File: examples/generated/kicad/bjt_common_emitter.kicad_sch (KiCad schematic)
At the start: 6 parts, among them Q1 2N3904

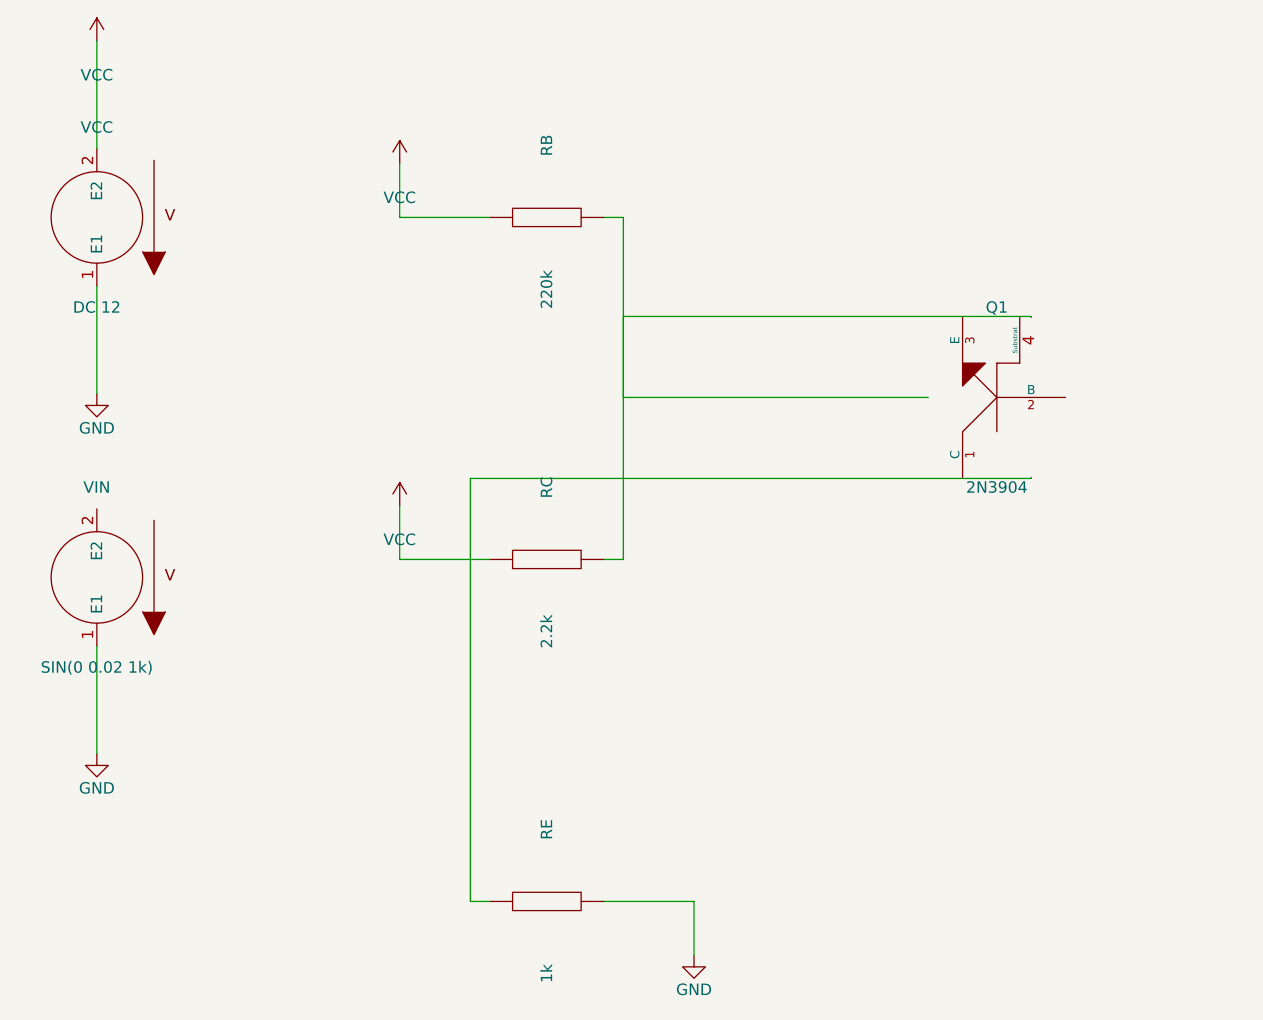
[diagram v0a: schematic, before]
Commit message: Attempt to fix more terminal issues.
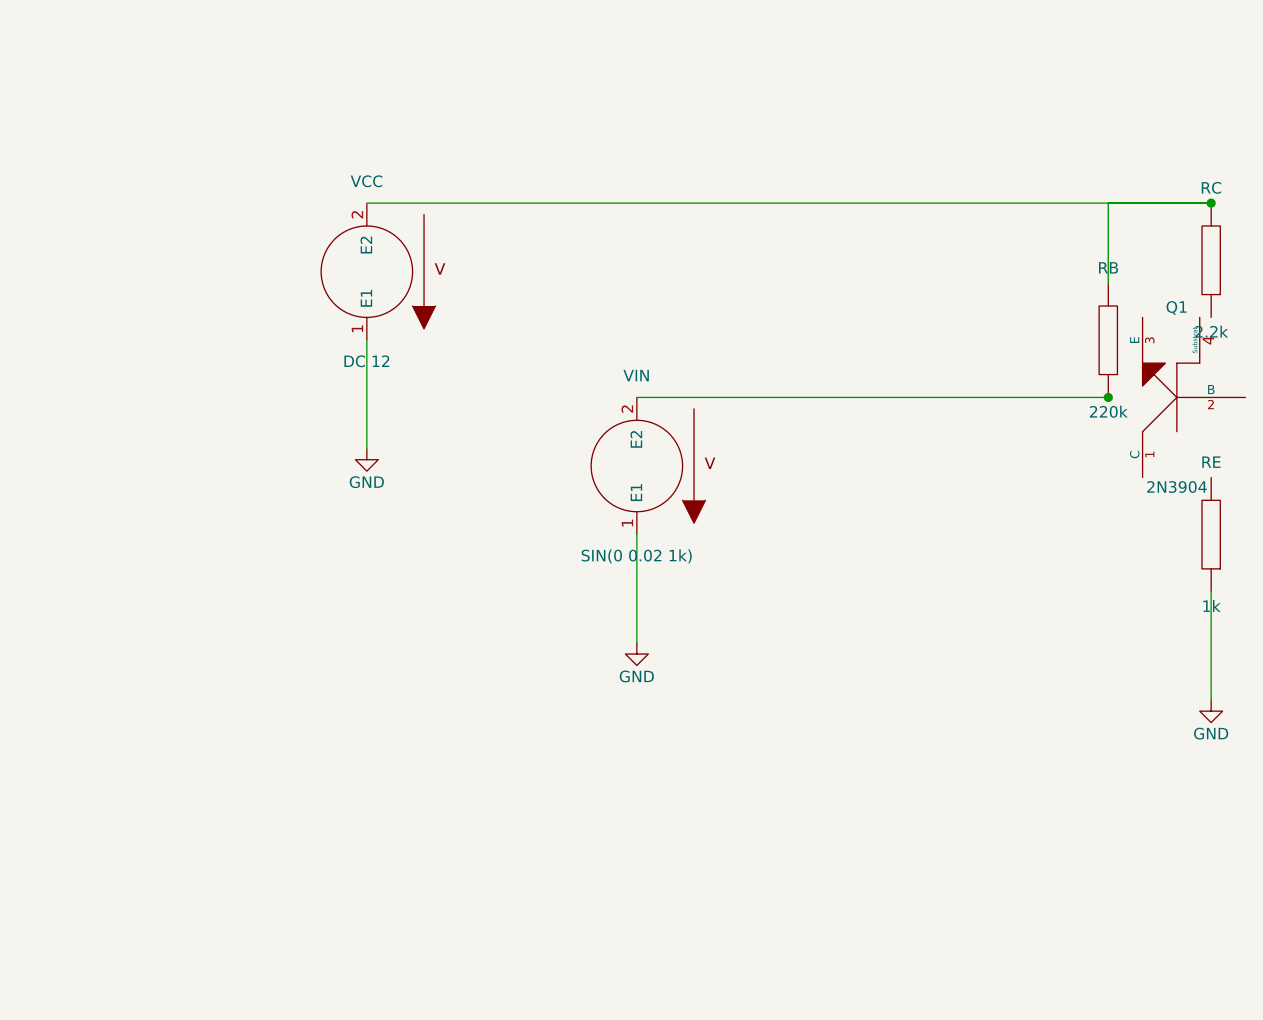
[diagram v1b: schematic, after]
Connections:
- net GND: now also RE.1; no longer RE.2
- net at RB.2, RC.2: now also VCC.2 (E2)
- net at VIN.2 (E2): now also RB.1
- removed net VCC: RB.1, RC.1, VCC.2 (E2)
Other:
- moved on the sheet: Q1, RB, RC, RE, VCC, VIN
